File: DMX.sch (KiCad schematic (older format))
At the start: 7 parts, among them U10 ST485CDR

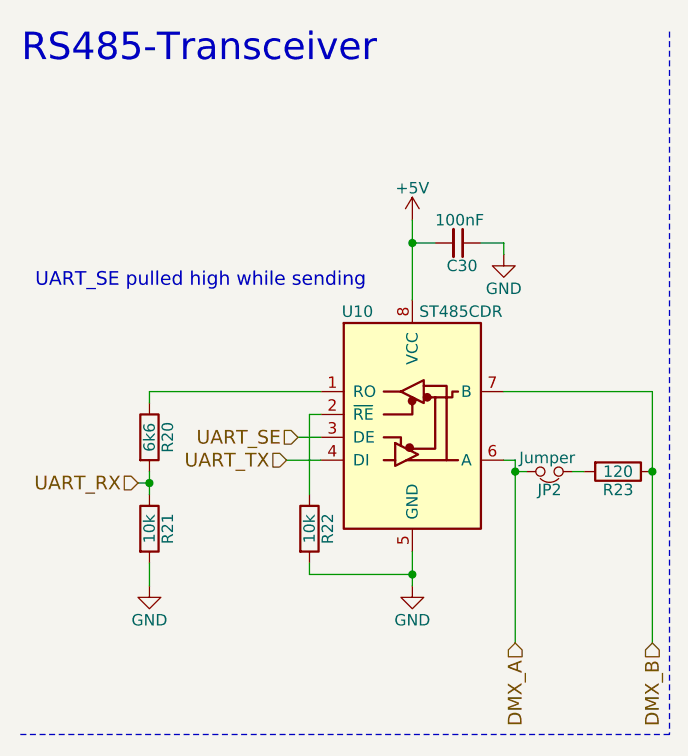
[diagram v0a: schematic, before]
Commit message: Added Component-Associations (about 10% remaining)
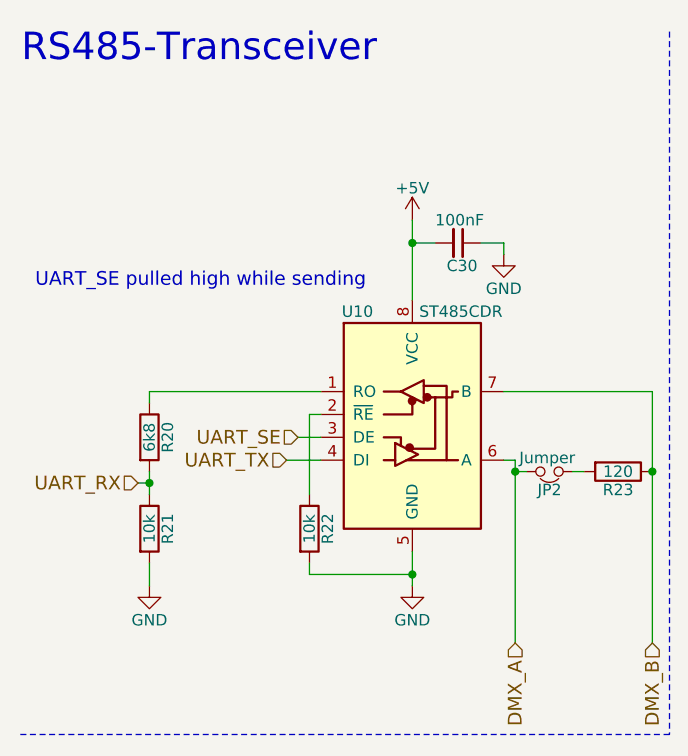
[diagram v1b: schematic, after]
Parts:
- C30: Buy (none) -> https://www.digikey.com/product-detail/en/kemet/C0603C104M5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
- R20: value 6k6 -> 6k8; Buy (none) -> https://www.digikey.com/product-detail/en/yageo/RC0603JR-07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
- R21, R22: Buy (none) -> https://www.digikey.com/product-detail/en/yageo/RC0603FR-07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
- R23: footprint Resistors_SMD:R_0603 -> Resistors_SMD:R_1206; Buy (none) -> https://www.digikey.com/product-detail/en/yageo/RC1206FR-07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
- U10: Buy (none) -> https://www.digikey.com/product-detail/en/stmicroelectronic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
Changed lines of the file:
@@
 F 2 "Housings_SOIC:SOIC-8_3.9x4.9mm_Pitch1.27mm" H 2200 1450 50  0001 C CNN
 F 3 "http://www.st.com/content/ccc/resource/technical/document/datasheet/4b/81/a8/cd/8a/72/47/82/CD00002183.pdf/files/CD00002183.pdf/jcr:content/translations/en.CD00002183.pdf" H 2200 2200 50  0001 C CNN
+F 4 "https://www.digikey.com/product-detail/en/stmicroelectronics/ST485CDR/497-3734-1-ND/686452" H 2200 2150 50  0001 C CNN "Buy"
 	1    2200 2150
 	1    0    0    -1
@@
 F 2 "Capacitors_SMD:C_0603" H 2400 1400 50  0001 C CNN
 F 3 "" H 2400 1400 50  0001 C CNN
+F 4 "https://www.digikey.com/product-detail/en/kemet/C0603C104M5RACTU/399-7845-1-ND/3471568" V 2400 1400 50  0001 C CNN "Buy"
 	1    2400 1400
 	0    1    1    0
@@
 P 1050 2250
 F 0 "R20" V 1130 2250 50  0000 C CNN
-F 1 "6k6" V 1050 2250 50  0000 C CNN
+F 1 "6k8" V 1050 2250 50  0000 C CNN
 F 2 "Resistors_SMD:R_0603" V 980 2250 50  0001 C CNN
 F 3 "" H 1050 2250 50  0001 C CNN
+F 4 "https://www.digikey.com/product-detail/en/yageo/RC0603JR-076K8L/311-6.8KGRCT-ND/729760" V 1050 2250 50  0001 C CNN "Buy"
 	1    1050 2250
 	1    0    0    -1
@@
 F 2 "Resistors_SMD:R_0603" V 980 2650 50  0001 C CNN
 F 3 "" H 1050 2650 50  0001 C CNN
+F 4 "https://www.digikey.com/product-detail/en/yageo/RC0603FR-0710KL/311-10.0KHRCT-ND/729827" V 1050 2650 50  0001 C CNN "Buy"
 	1    1050 2650
 	1    0    0    -1
@@
 F 2 "Resistors_SMD:R_0603" V 1680 2650 50  0001 C CNN
 F 3 "" H 1750 2650 50  0001 C CNN
+F 4 "https://www.digikey.com/product-detail/en/yageo/RC0603FR-0710KL/311-10.0KHRCT-ND/729827" V 1750 2650 50  0001 C CNN "Buy"
 	1    1750 2650
 	1    0    0    -1
@@
 F 0 "R23" V 3180 2400 50  0000 C CNN
 F 1 "120" V 3100 2400 50  0000 C CNN
-F 2 "Resistors_SMD:R_0603" V 3030 2400 50  0001 C CNN
+F 2 "Resistors_SMD:R_1206" V 3030 2400 50  0001 C CNN
 F 3 "" H 3100 2400 50  0001 C CNN
+F 4 "https://www.digikey.com/product-detail/en/yageo/RC1206FR-07120RL/311-120FRCT-ND/731470" V 3100 2400 50  0001 C CNN "Buy"
 	1    3100 2400
 	0    1    1    0
